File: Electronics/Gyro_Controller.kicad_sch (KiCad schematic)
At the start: 35 parts, among them J3 SWCLK SWD, SW3 SW_Push, SW4 ~{USB_BOOT}, U7 W25Q32JVZP, U8 RP2040, Y2 ABM8-272-T3

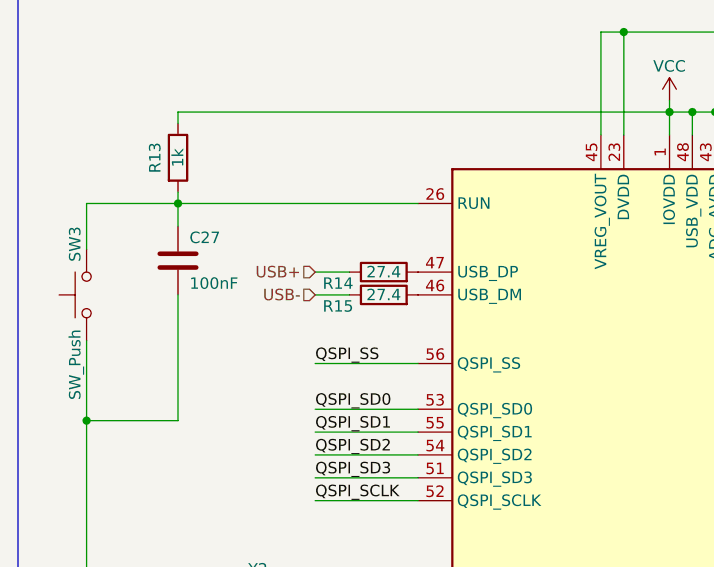
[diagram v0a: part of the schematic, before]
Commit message: power + usb
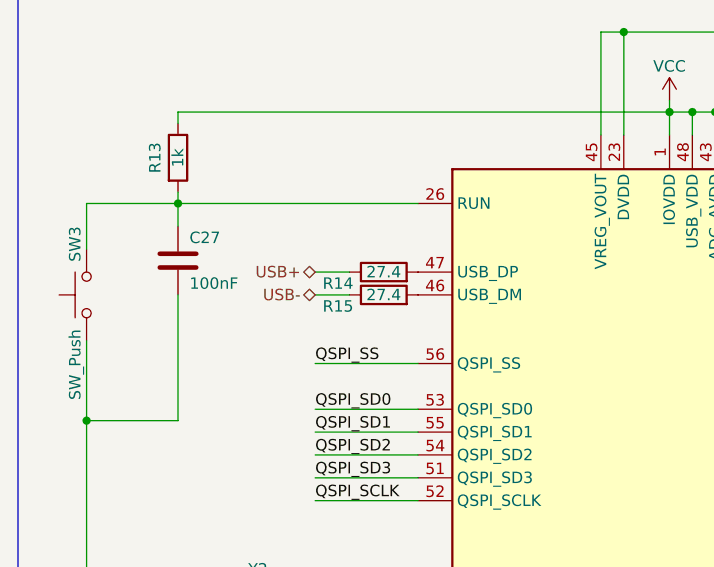
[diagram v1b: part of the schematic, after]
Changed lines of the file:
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@@
     (effects (font (size 1.27 1.27)) (justify right bottom))
   )
-  (hierarchical_label "USB+" (shape input) (at 48.26 49.53 180) (fields_autoplaced)
+  (hierarchical_label "USB+" (shape bidirectional) (at 48.26 49.53 180) (fields_autoplaced)
     (effects (font (size 1.27 1.27)) (justify right))
   )
@@
     (effects (font (size 1.27 1.27)) (justify left))
   )
-  (hierarchical_label "USB-" (shape input) (at 48.26 52.07 180) (fields_autoplaced)
+  (hierarchical_label "USB-" (shape bidirectional) (at 48.26 52.07 180) (fields_autoplaced)
     (effects (font (size 1.27 1.27)) (justify right))
   )
